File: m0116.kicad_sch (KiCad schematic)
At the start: 262 parts, among them J1 Conn_01x05, J2 Conn_01x04_MountingPin, J3 Conn_01x04_MountingPin, J4 Conn_01x04, J7 Conn_01x05, Q1 Q_PMOS_GSD AO3401A, Q2 Q_NMOS_GSD 2N7002, Q3 Q_NMOS_GSD 2N7002, Q4 2N3904, SW1 SW_Push, U1 XC6206P332MR, U2 74AHCT1G125, U3 STM32F411RETx, U4 24LC64, U5 USBLC6-2SC6, Y1 8MHz

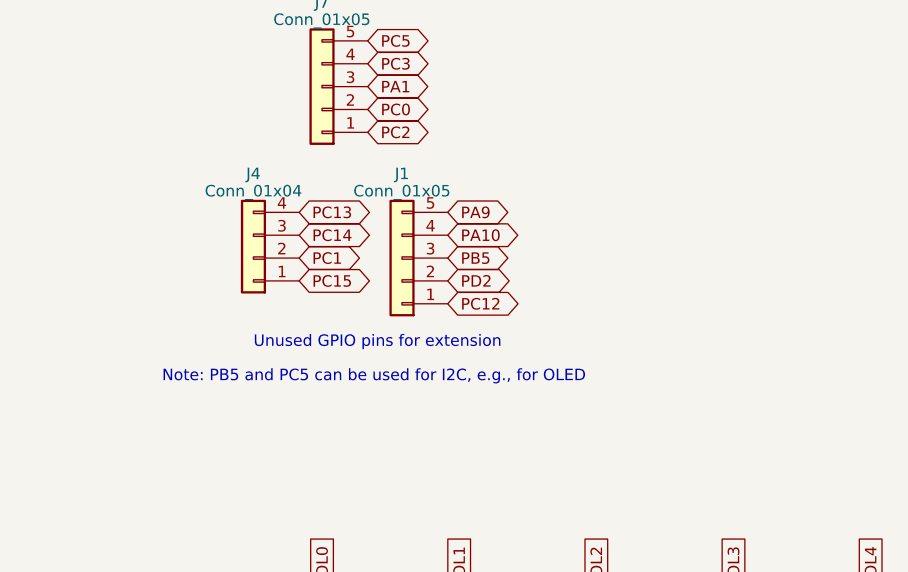
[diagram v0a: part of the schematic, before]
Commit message: updates
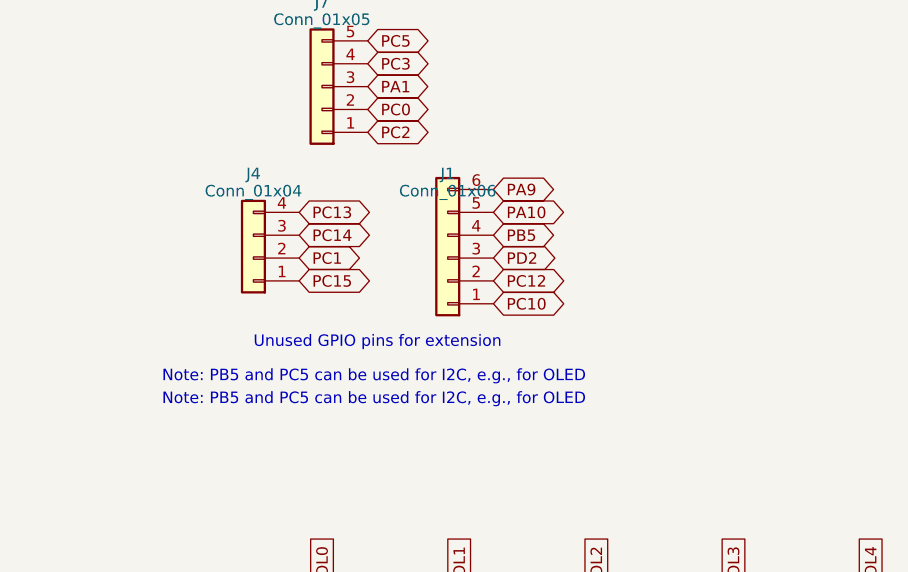
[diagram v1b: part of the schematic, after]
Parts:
- J1: value Conn_01x05 -> Conn_01x06; footprint Connector_PinHeader_1.27mm:PinHeader_1x05_P1.27mm_Vertical -> Connector_PinHeader_1.27mm:PinHeader_1x06_P1.27mm_Vertical; symbol Connector_Generic:Conn_01x05 -> Connector_Generic:Conn_01x06
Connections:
- net PA10: now also J1.5 (Pin_5); no longer J1.4 (Pin_4)
- net PA9: now also J1.6 (Pin_6); no longer J1.5 (Pin_5)
- net PB5: now also J1.4 (Pin_4); no longer J1.3 (Pin_3)
- net PC10: now also J1.1 (Pin_1)
- net PC12: now also J1.2 (Pin_2); no longer J1.1 (Pin_1)
- net PD2: now also J1.3 (Pin_3); no longer J1.2 (Pin_2)
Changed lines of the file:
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@@
     (effects (font (size 1.27 1.27)) (justify left bottom))
   )
+  (text "Note: PB5 and PC5 can be used for I2C, e.g., for OLED"
+    (at 22.86 237.49 0)
+    (effects (font (size 1.27 1.27)) (justify left bottom))
+  )
   (text "One per VDD pin" (at 181.61 27.305 0)
     (effects (font (size 1.27 1.27)) (justify left bottom))
@@
     )
   )
-  (global_label "PB5" (shape bidirectional) (at 54.61 220.98 0)
+  (global_label "PB5" (shape bidirectional) (at 59.69 218.44 0)
     (effects (font (size 1.27 1.27)) (justify left))
-    (property "Intersheetrefs" "${INTERSHEET_REFS}" (at 54.61 220.98 0)
+    (property "Intersheetrefs" "${INTERSHEET_REFS}" (at 59.69 218.44 0)
       (effects (font (size 1.27 1.27)) hide)
     )
@@
     )
   )
-  (global_label "PD2" (shape bidirectional) (at 54.61 223.52 0)
+  (global_label "PD2" (shape bidirectional) (at 59.69 220.98 0)
     (effects (font (size 1.27 1.27)) (justify left))
-    (property "Intersheetrefs" "${INTERSHEET_REFS}" (at 54.61 223.52 0)
+    (property "Intersheetrefs" "${INTERSHEET_REFS}" (at 59.69 220.98 0)
       (effects (font (size 1.27 1.27)) hide)
     )
@@
     )
   )
-  (global_label "PA10" (shape bidirectional) (at 54.61 218.44 0)
+  (global_label "PA10" (shape bidirectional) (at 59.69 215.9 0)
     (effects (font (size 1.27 1.27)) (justify left))
-    (property "Intersheetrefs" "${INTERSHEET_REFS}" (at 54.61 218.44 0)
+    (property "Intersheetrefs" "${INTERSHEET_REFS}" (at 59.69 215.9 0)
       (effects (font (size 1.27 1.27)) hide)
     )
@@
     )
   )
-  (global_label "PC12" (shape bidirectional) (at 54.61 226.06 0)
+  (global_label "PC12" (shape bidirectional) (at 59.69 223.52 0)
     (effects (font (size 1.27 1.27)) (justify left))
-    (property "Intersheetrefs" "${INTERSHEET_REFS}" (at 54.61 226.06 0)
+    (property "Intersheetrefs" "${INTERSHEET_REFS}" (at 59.69 223.52 0)
       (effects (font (size 1.27 1.27)) hide)
     )
@@
     )
   )
-  (global_label "PA9" (shape bidirectional) (at 54.61 215.9 0)
+  (global_label "PA9" (shape bidirectional) (at 59.69 213.36 0)
     (effects (font (size 1.27 1.27)) (justify left))
-    (property "Intersheetrefs" "${INTERSHEET_REFS}" (at 54.61 215.9 0)
+    (property "Intersheetrefs" "${INTERSHEET_REFS}" (at 59.69 213.36 0)
       (effects (font (size 1.27 1.27)) hide)
     )
@@
     )
   )
+  (global_label "PC10" (shape bidirectional) (at 59.69 226.06 0)
+    (effects (font (size 1.27 1.27)) (justify left))
+    (property "Intersheetrefs" "${INTERSHEET_REFS}" (at 59.69 226.06 0)
+      (effects (font (size 1.27 1.27)) hide)
+    )
+  )
   (global_label "COL7" (shape input) (at 151.13 259.08 90) (fields_autoplaced)
     (effects (font (size 1.27 1.27)) (justify left))
@@
     )
   )
-  (symbol (lib_id "Connector_Generic:Conn_01x05") (at 49.53 220.98 180) (unit 1)
+  (symbol (lib_id "Connector_Generic:Conn_01x06") (at 54.61 220.98 180) (unit 1)
     (in_bom yes) (on_board yes) (dnp no) (fields_autoplaced)
-    (property "Reference" "J1" (at 49.53 211.6201 0)
+    (property "Reference" "J1" (at 54.61 211.6201 0)
       (effects (font (size 1.27 1.27)))
     )
-    (property "Value" "Conn_01x05" (at 49.53 213.5411 0)
+    (property "Value" "Conn_01x06" (at 54.61 213.5411 0)
       (effects (font (size 1.27 1.27)))
     )
-    (property "Footprint" "Connector_PinHeader_1.27mm:PinHeader_1x05_P1.27mm_Vertical" (at 49.53 220.98 0)
+    (property "Footprint" "Connector_PinHeader_1.27mm:PinHeader_1x06_P1.27mm_Vertical" (at 54.61 220.98 0)
       (effects (font (size 1.27 1.27)) hide)
     )
-    (property "Datasheet" "~" (at 49.53 220.98 0)
+    (property "Datasheet" "~" (at 54.61 220.98 0)
       (effects (font (size 1.27 1.27)) hide)
     )
@@
     (pin "4")
     (pin "5")
+    (pin "6")
     (instances
       (project "m0116"
